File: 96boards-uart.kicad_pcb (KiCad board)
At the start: 2 copper layers, 41 x 14 mm, 33 parts, among them J1 CONN_02X03, J2 CONN_20X2, J3 CONN_01X02, Q1 S8050, SW1 RST, U1 REG_1.8V, U2 FT230XS-R

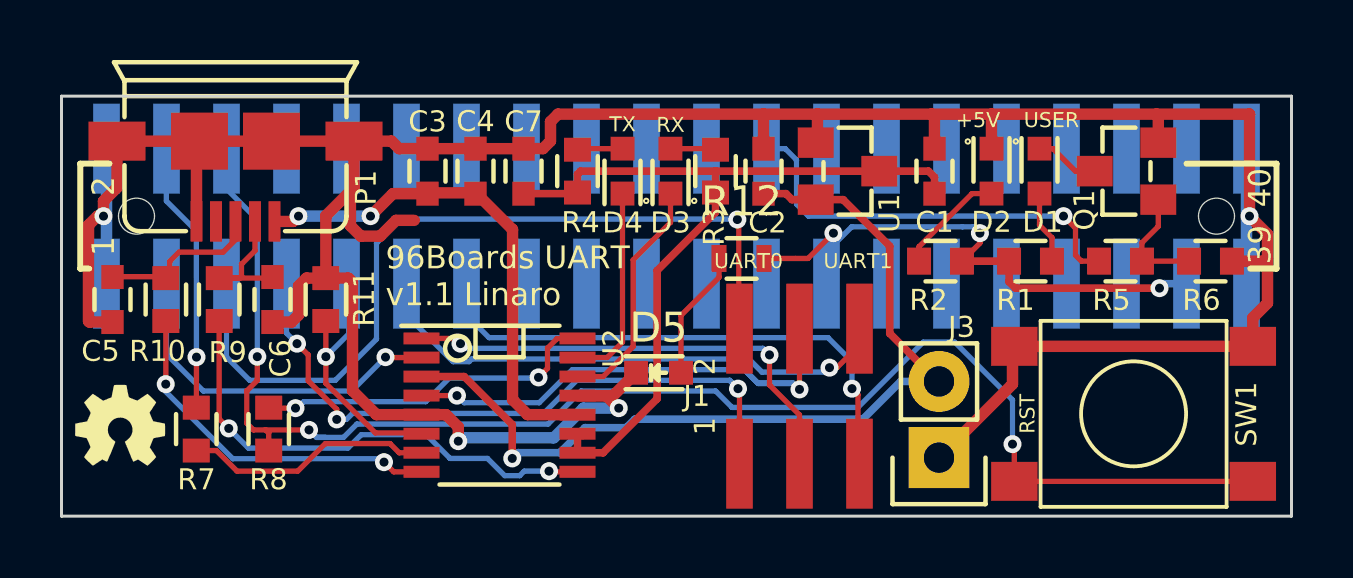
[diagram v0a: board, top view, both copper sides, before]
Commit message: PCB Layout
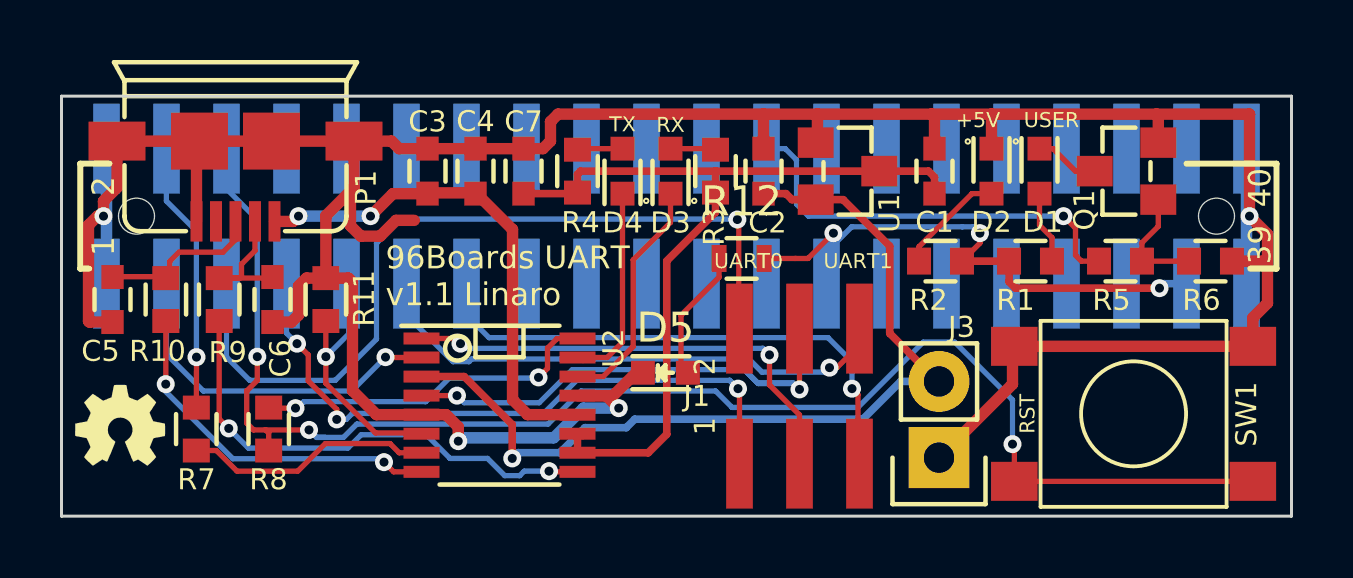
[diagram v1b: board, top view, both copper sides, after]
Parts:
- moved D5 0.23 mm to (120.1, 109.2)
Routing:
- net +3V3_FTDI: track 27.5 -> 28.4 mm
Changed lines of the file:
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@@
   (general
     (links 74)
-    (no_connects 4)
-    (area 99.949999 99.949999 141.050001 114.050001)
+    (no_connects 0)
+    (area 95.177986 97.2847 141.050001 114.050001)
     (thickness 1.6)
     (drawings 20)
@@
     (34 B.Paste user)
     (35 F.Paste user)
-    (36 B.SilkS user hide)
+    (36 B.SilkS user)
     (37 F.SilkS user)
-    (38 B.Mask user hide)
-    (39 F.Mask user hide)
-    (40 Dwgs.User user hide)
-    (41 Cmts.User user hide)
-    (42 Eco1.User user hide)
-    (43 Eco2.User user hide)
-    (44 Edge.Cuts user hide)
+    (38 B.Mask user)
+    (39 F.Mask user)
+    (40 Dwgs.User user)
+    (41 Cmts.User user)
+    (42 Eco1.User user)
+    (43 Eco2.User user)
+    (44 Edge.Cuts user)
   )
   (setup
@@
   )
   (module LEDs:LED-0603 (layer F.Cu)
-    (at 119.9007 109.22)
+    (at 120.1293 109.22)
     (descr "LED 0603 smd package")
     (tags "LED led 0603 SMD smd SMT smt smdled SMDLED smtled SMTLED")
@@
   (segment (start 118.7 101.7507) (end 117.2007 101.7507) (width 0.1778) (layer F.Cu) (net 26) (status 30))
   (segment (start 117.2007 101.7507) (end 117.2 101.75) (width 0.1778) (layer F.Cu) (net 26) (status 30))
-  (segment (start 117.2 111.8875) (end 118.054 111.8875) (width 0.254) (layer F.Cu) (net 27))
-  (segment (start 118.054 111.8875) (end 119.854981 110.086519) (width 0.254) (layer F.Cu) (net 27))
-  (segment (start 119.854981 105.814019) (end 121.8 103.869) (width 0.254) (layer F.Cu) (net 27))
+  (segment (start 117.2 111.8875) (end 119.557302 111.8875) (width 0.254) (layer F.Cu) (net 27))
+  (segment (start 119.557302 111.8875) (end 120.175019 111.269783) (width 0.254) (layer F.Cu) (net 27))
+  (segment (start 120.175019 111.269783) (end 120.175019 105.493981) (width 0.254) (layer F.Cu) (net 27))
+  (segment (start 120.175019 105.493981) (end 121.8 103.869) (width 0.254) (layer F.Cu) (net 27))
   (segment (start 121.8 103.869) (end 121.8 103.215) (width 0.254) (layer F.Cu) (net 27))
-  (segment (start 119.854981 110.086519) (end 119.854981 105.814019) (width 0.254) (layer F.Cu) (net 27))
   (segment (start 129.1 103.25) (end 129.1 102.7) (width 0.254) (layer F.Cu) (net 27) (status 10))
   (segment (start 128.9 102.5) (end 127.19822 102.5) (width 0.254) (layer F.Cu) (net 27) (status 20))
